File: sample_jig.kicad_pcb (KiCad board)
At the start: 2 copper layers, 50 x 50 mm, 25 parts

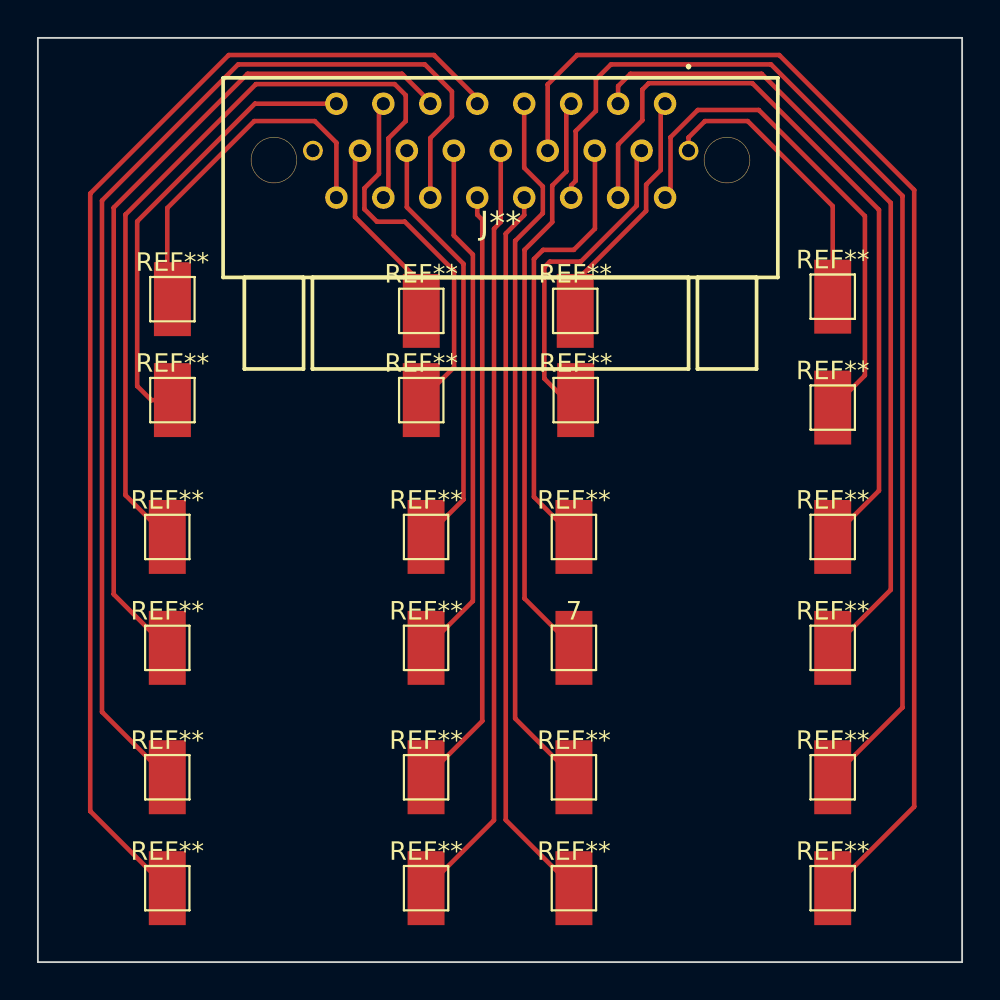
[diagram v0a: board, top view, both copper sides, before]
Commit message: finalized version of the board for cirexx
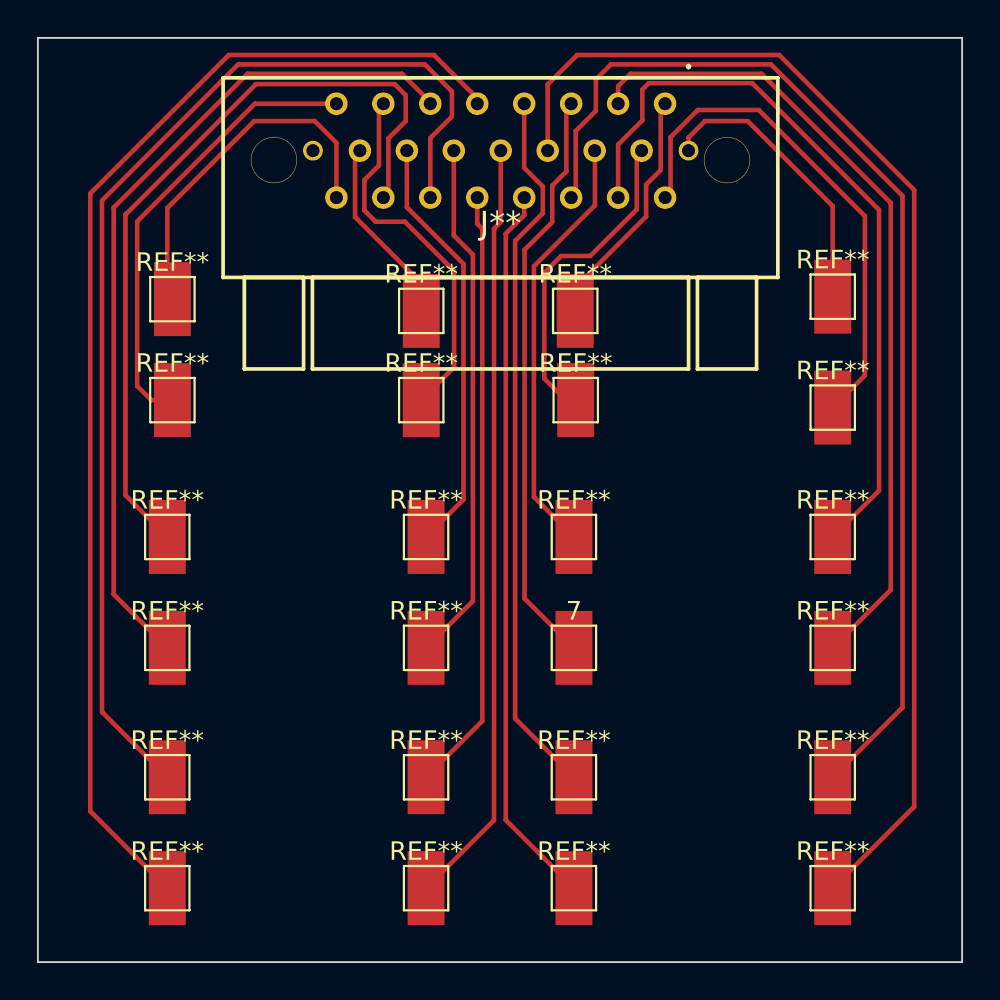
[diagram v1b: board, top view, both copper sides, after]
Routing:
- net (no net): track 835.4 -> 834.4 mm
